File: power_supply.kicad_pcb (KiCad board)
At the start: 2 copper layers, 85 x 56 mm, 24 parts, among them J1 12v, 2A, J2 Screw_Terminal_01x02, J3 Fan, J4 Conn_01x05, M1 U3V70F5, M2 D24V50F5, U1 ALD910027, U2 MCP9700A-E_TO, U3 PIC12F1840-ISN

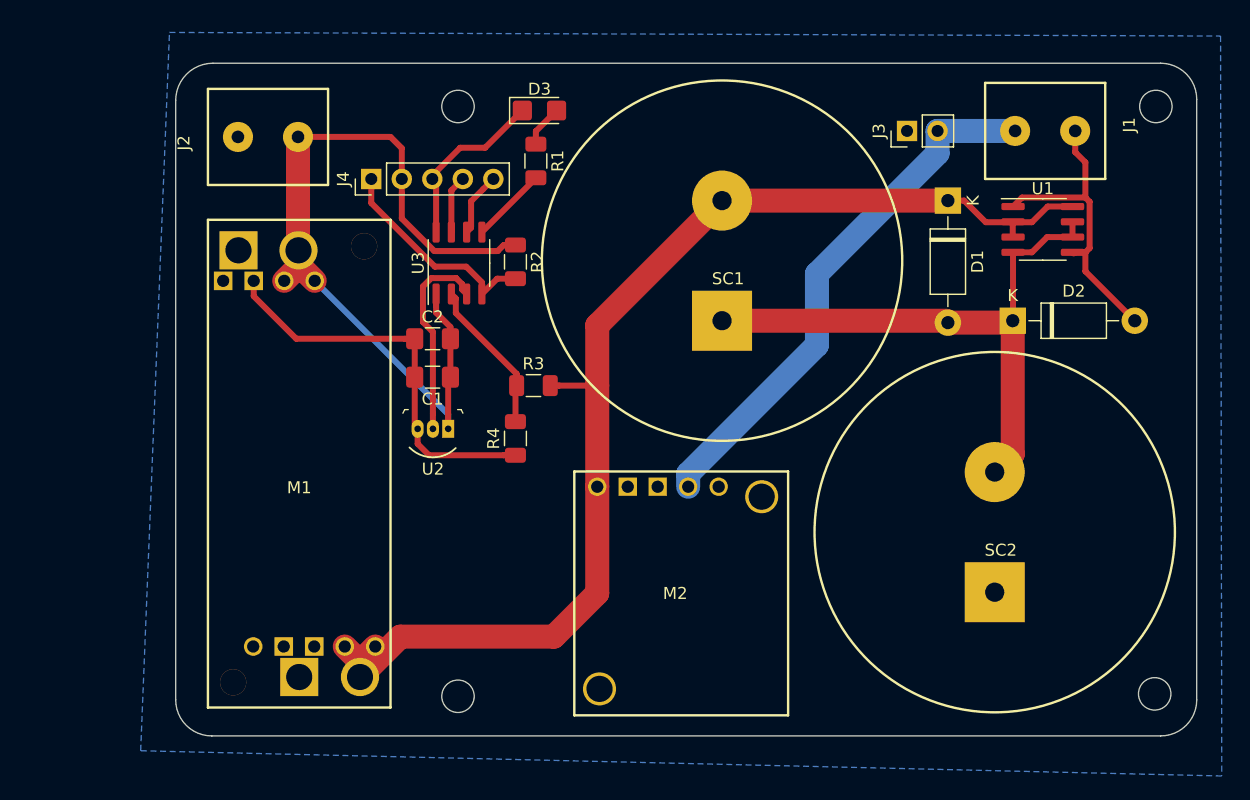
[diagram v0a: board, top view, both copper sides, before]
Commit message: Version 1.0 includes fixes/changes and FRAM support
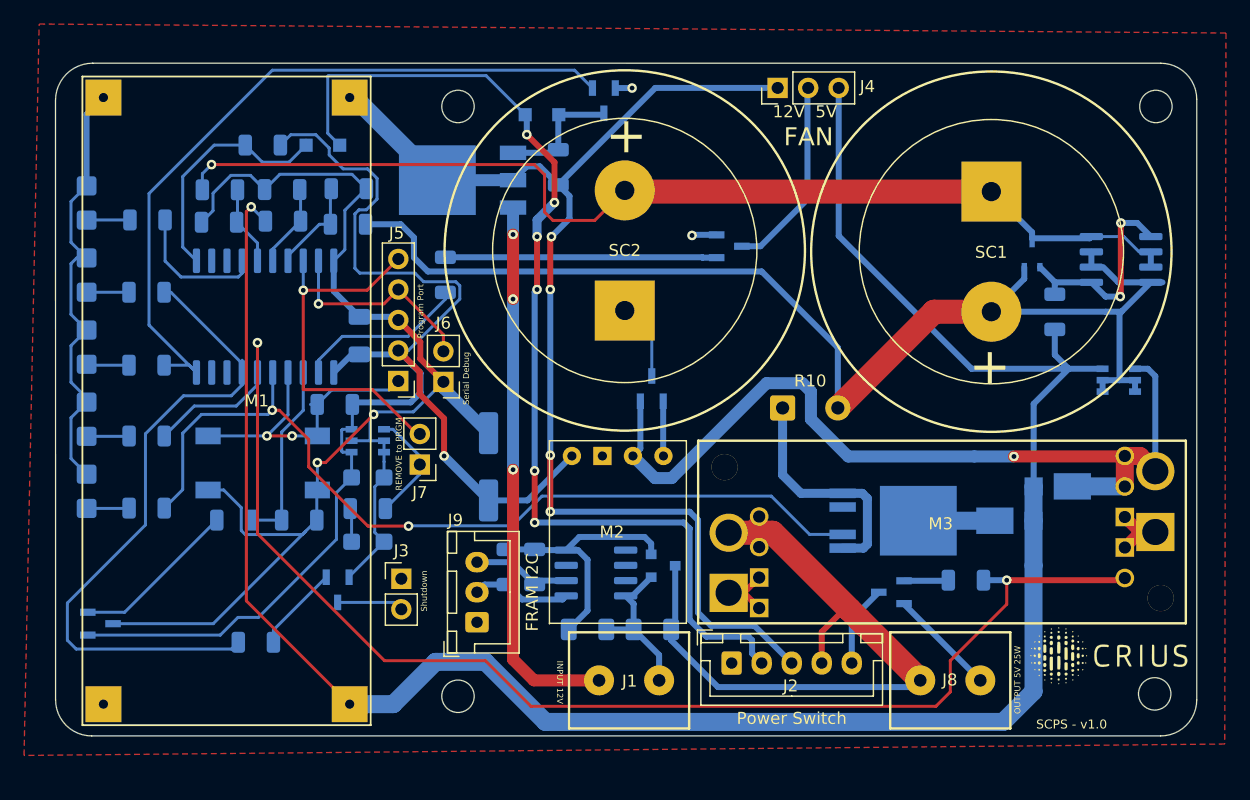
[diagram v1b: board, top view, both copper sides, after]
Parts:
- added C3: 2.2uF Tant, Capacitor_Tantalum_SMD:CP_EIA-3216-18_Kemet-A, B.Cu at (118.4, 115.8)
- added C4: 2.2uF Tant, Capacitor_Tantalum_SMD:CP_EIA-3216-18_Kemet-A, B.Cu at (118.4, 121.2)
- added C5: 1uF, Capacitor_SMD:C_1206_3216Metric_Pad1.33x1.80mm_HandSolder, B.Cu at (136.7, 128.5)
- added C6: 1uF, Capacitor_SMD:C_1206_3216Metric_Pad1.33x1.80mm_HandSolder, B.Cu at (142.1, 128.5)
- added D10: PWRUP, Diode_SMD:D_1206_3216Metric_Castellated, B.Cu at (95.0, 111.0)
- added D4: FAULT, Diode_SMD:D_1206_3216Metric_Castellated, B.Cu at (95.0, 117.0)
- added D5: V8PAM10S, Footprint_Library:DO-221BC, B.Cu at (171.8, 119.5)
- added D6: MAINPWR, Diode_SMD:D_1206_3216Metric_Castellated, B.Cu at (95.0, 105.0)
- added D7: BAT54SW, Package_TO_SOT_SMD:SOT-323_SC-70, B.Cu at (173.7, 97.3)
- added D8: Activity, Diode_SMD:D_1206_3216Metric_Castellated, B.Cu at (95.0, 93.0)
- added D9: V8PAM10S, Footprint_Library:DO-221BC, B.Cu at (175.8, 116.6)
- added G***: LOGO, Crius:Crius_logo_36x9mm, B.Cu at (170.4, 86.8)
- added G***: LOGO, Crius:Crius_logo_20x5mm, F.Cu at (180.1, 130.7)
- added J5: Program, Connector_PinHeader_2.54mm:PinHeader_1x05_P2.54mm_Vertical, F.Cu at (121.0, 107.8)
- added J6: Serial Debug, Connector_PinHeader_2.54mm:PinHeader_1x02_P2.54mm_Vertical, F.Cu at (124.7, 107.9)
- added J7: REMOVE to PRGM, Connector_PinHeader_2.54mm:PinHeader_1x02_P2.54mm_Vertical, F.Cu at (122.7, 114.8)
- added J8: 5V 25W, Connectors:Screw_Terminal_2Pin, F.Cu at (166.9, 132.7)
- added J9: FRAM I2C, Connector_JST:JST_XH_B3B-XH-A_1x03_P2.50mm_Vertical, F.Cu at (127.5, 127.9)
- added M3: U3V70F5, Pololu:U3V70F5, F.Cu at (166.2, 120.4)
- added Q1: BSS806, digikey-footprints:SOT-23-3, B.Cu at (138.1, 84.5)
- added Q2: BSS806, digikey-footprints:SOT-23-3, B.Cu at (148.5, 96.6)
- added Q3: SPD18P06PGBTMA1, Package_TO_SOT_SMD:TO-252-3_TabPin2, B.Cu at (126.3, 91.1)
- added Q4: BSS806, digikey-footprints:SOT-23-3, B.Cu at (162.0, 125.4)
- added Q5: BSS806, digikey-footprints:SOT-23-3, B.Cu at (115.9, 125.2)
- added Q6: SQ3495-EV, digikey-footprints:SOT-23-6, B.Cu at (180.9, 107.8)
- added R10: 1R 25W, Connector_Wire:SolderWire-0.5sqmm_1x02_P4.6mm_D0.9mm_OD2.1mm, F.Cu at (152.9, 110.1)
- added R11: 1k, Resistor_SMD:R_1206_3216Metric, B.Cu at (100.0, 106.5)
- added R12: 10k, Resistor_SMD:R_1206_3216Metric, B.Cu at (109.7, 88.2)
- added R13: 9k 0.1%, Resistor_SMD:R_1206_3216Metric, B.Cu at (106.1, 91.9)
- added R14: 1k, Resistor_SMD:R_1206_3216Metric, B.Cu at (100.1, 94.4)
- added R15: 9k 0.1%, Resistor_SMD:R_1206_3216Metric, B.Cu at (111.3, 94.5)
- added R16: 1k 0.1%, Resistor_SMD:R_1206_3216Metric, B.Cu at (106.0, 94.6)
- added R17: 9k 0.1%, Resistor_SMD:R_1206_3216Metric, B.Cu at (116.8, 94.8)
- added R18: 10k, Resistor_SMD:R_1206_3216Metric, B.Cu at (175.6, 102.1)
- added R19: 1k 0.1%, Resistor_SMD:R_1206_3216Metric, B.Cu at (111.3, 91.9)
- added R20: 1k 0.1%, Resistor_SMD:R_1206_3216Metric, B.Cu at (116.8, 91.8)
- added R21: 1k, Resistor_SMD:R_1206_3216Metric, B.Cu at (100.0, 112.4)
- added R22: 50, Resistor_SMD:R_1206_3216Metric, B.Cu at (118.4, 118.4)
- added R23: 10k, Resistor_SMD:R_1206_3216Metric, B.Cu at (132.3, 123.3)
- added R24: 10k, Resistor_SMD:R_1206_3216Metric, B.Cu at (130.0, 123.3)
- added R5: 1k, Resistor_SMD:R_1206_3216Metric, B.Cu at (168.2, 124.4)
- added R6: 1k, Resistor_SMD:R_1206_3216Metric, B.Cu at (100.0, 118.4)
- added R7: 1k 0.1%, Resistor_SMD:R_1206_3216Metric, B.Cu at (107.3, 119.4)
- added R8: 1k 0.1%, Resistor_SMD:R_1206_3216Metric, B.Cu at (112.7, 119.4)
- added R9: 10k, Resistor_SMD:R_1206_3216Metric, B.Cu at (115.7, 109.8)
- added S1: RESET, digikey-footprints:Switch_Tactile_SMD_6x6mm, B.Cu at (109.7, 114.6)
- added U4: PIC16F1709, Package_SO:SOIC-20W_7.5x12.8mm_P1.27mm, B.Cu at (109.9, 102.5)
- added U5: MCP111-195, digikey-footprints:SOT-23-3, B.Cu at (142.1, 108.5)
- added U6: MB85RC1MT, Package_SO:SOIC-8_3.9x4.9mm_P1.27mm, B.Cu at (137.4, 123.8)
- added U7: MCP1700-3302E_SOT23, Package_TO_SOT_SMD:SOT-23, B.Cu at (143.0, 123.2)
- added VRef1: MCP1501-6Pin, digikey-footprints:SOT-23-6, B.Cu at (118.4, 112.8)
- C1: value .1 -> 100uF; footprint Capacitor_SMD:C_1206_3216Metric_Pad1.42x1.75mm_HandSolder -> Capacitor_SMD:CP_Elec_6.3x5.2; moved to B.Cu
- C2: footprint Capacitor_SMD:C_1206_3216Metric_Pad1.42x1.75mm_HandSolder -> Capacitor_SMD:C_1206_3216Metric_Pad1.33x1.80mm_HandSolder; moved to B.Cu
- D1, D2: value 1N5817 -> 1N914; footprint Diode_THT:D_DO-41_SOD81_P10.16mm_Horizontal -> Diode_SMD:D_SOD-123F; moved to B.Cu
- D3: value LED -> ShutDown; moved to B.Cu
- J1: value 12v, 2A -> 12v, 0.5A nominal, 5A Surge
- J2: value Screw_Terminal_01x02 -> Power Switch; footprint Connectors:Screw_Terminal_2Pin -> Connector_JST:JST_XH_B5B-XH-A_1x05_P2.50mm_Vertical
- J3: value Fan -> Shutdown
- J4: value Conn_01x05 -> 12V 5V; footprint Connector_PinHeader_2.54mm:PinHeader_1x05_P2.54mm_Vertical -> Connector_PinHeader_2.54mm:PinHeader_1x03_P2.54mm_Vertical
- M1: value U3V70F5 -> XL4015; footprint Pololu Regulators:U3V70F5 -> Footprint_Library:XL4015
- M2: value D24V50F5 -> U1V11F5; footprint Pololu Regulators:D24V50F5 -> Pololu:U1V11Fx
- R1: value 1k -> 10k; moved to B.Cu
- R2: value 10k -> 1k; moved to B.Cu
- R3, R4: moved to B.Cu
- SC1, SC2: value SuperCap -> 100F/200F; footprint SuperCaps:SCC-30mm -> SuperCaps:SCC-22-30mm
- U1: value ALD910027 -> MCP9700A; footprint Package_SO:SOIC-8_3.9x4.9mm_P1.27mm -> digikey-footprints:SOT-23-3; moved to B.Cu
- U2: value MCP9700A-E_TO -> BTS443P; footprint digikey-footprints:TO-92-3 -> Package_TO_SOT_SMD:TO-252-4; moved to B.Cu
- U3: value PIC12F1840-ISN -> ALD910027; footprint Package_SO:SO-8_3.9x4.9mm_P1.27mm -> Package_SO:SOIC-8_3.9x4.9mm_P1.27mm; moved to B.Cu
- moved U1 85.0 mm to (96.2, 128.0)
- moved J2 58.4 mm to (148.7, 131.3), turned to 0 degrees
- moved J1 57.4 mm to (140.2, 132.7)
- moved J3 56.2 mm to (121.2, 124.3), turned to 0 degrees
- moved U3 55.1 mm to (181.1, 97.7), turned to 0 degrees
- moved D1 52.2 mm to (114.7, 88.2), turned to 180 degrees
- moved D2 42.8 mm to (132.9, 85.7)
- moved D3 40.1 mm to (95.0, 99.0), turned to 270 degrees
- moved SC2 38.7 mm to (139.8, 97.0)
- moved R2 38.3 mm to (109.1, 129.6), turned to 0 degrees
- moved U2 37.8 mm to (162.1, 119.5), turned to 0 degrees
- moved J4 34.7 mm to (152.5, 83.4)
- moved R3 33.1 mm to (100.0, 100.4), turned to 180 degrees
- moved SC1 22.4 mm to (170.3, 97.0), turned to 180 degrees
- moved R4 14.8 mm to (124.9, 99.0)
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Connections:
- C1 pad 1: /5V -> Net-(C1-Pad1)
- C1 pad 2: /GND -> Net-(C1-Pad2)
- C2 pad 1: /GND -> Net-(C1-Pad2)
- C2 pad 2: /5V -> Net-(C1-Pad1)
- D1 pad 1: /2.5-5V -> Net-(D1-Pad1)
- D2 pad 1: Net-(D1-Pad2) -> Net-(D1-Pad1)
- D2 pad 2: /GND -> Net-(D2-Pad2)
- D3 pad 1: /GND -> Net-(C1-Pad2)
- J1 pad 1: /GND -> Net-(C1-Pad2)
- J1 pad 2: /12v -> Net-(J1-Pad2)
- J2 pad 1: /GND -> Net-(C1-Pad2)
- J2 pad 2: /5V -> Net-(D1-Pad1)
- J3 pad 1: /GND -> Net-(C1-Pad2)
- J3 pad 2: /12v -> Net-(J3-Pad2)
- J4 pad 1: Net-(J4-Pad1) -> Net-(J2-Pad3)
- J4 pad 2: /5V -> Net-(J4-Pad2)
- J4 pad 3: /GND -> Net-(D5-Pad2)
- M1 pad 1: Net-(M1-Pad1) -> Net-(J2-Pad3)
- M1 pad 2: /GND -> Net-(C1-Pad2)
- M1 pad 3: /GND -> Net-(C1-Pad2)
- M1 pad 4: /GND -> Net-(D5-Pad2)
- M2 pad 1: Net-(M2-Pad1) -> Net-(C1-Pad1)
- M2 pad 2: /12v -> Net-(C1-Pad2)
- M2 pad 3: /GND -> Net-(D9-Pad1)
- M2 pad 4: /GND -> Net-(M2-Pad4)
- R1 pad 1: Net-(D3-Pad2) -> Net-(D2-Pad2)
- R1 pad 2: Net-(R1-Pad2) -> Net-(J2-Pad3)
- R2 pad 1: /5V -> Net-(R2-Pad1)
- R2 pad 2: Net-(J4-Pad1) -> Net-(Q5-Pad1)
- R3 pad 1: Net-(R3-Pad1) -> Net-(R2-Pad1)
- R3 pad 2: /2.5-5V -> Net-(D3-Pad2)
- R4 pad 1: /GND -> Net-(R4-Pad1)
- R4 pad 2: Net-(R3-Pad1) -> Net-(Q2-Pad1)
- SC1 pad 1: Net-(D1-Pad2) -> Net-(D7-Pad3)
- SC1 pad 2: /2.5-5V -> Net-(D7-Pad2)
- SC2 pad 1: /GND -> Net-(C1-Pad2)
- SC2 pad 2: Net-(D1-Pad2) -> Net-(D7-Pad3)
- U1 pad 1: /GND -> Net-(C1-Pad1)
- U1 pad 2: /2.5-5V -> Net-(R7-Pad2)
- U1 pad 3: /2.5-5V -> Net-(C1-Pad2)
- U2 pad 1: /5V -> Net-(R10-Pad1)
- U2 pad 2: Net-(U2-Pad2) -> Net-(R6-Pad1)
- U2 pad 3: /GND -> Net-(D5-Pad1)
- U3 pad 1: /5V -> Net-(C1-Pad2)
- U3 pad 2: Net-(R3-Pad1) -> Net-(D7-Pad2)
- U3 pad 3: Net-(U2-Pad2) -> Net-(D7-Pad2)
- U3 pad 4: Net-(J4-Pad1) -> Net-(D7-Pad3)
- U3 pad 5: Net-(R1-Pad2) -> Net-(C1-Pad2)
- U3 pad 6: Net-(J4-Pad5) -> Net-(D7-Pad3)
- U3 pad 7: Net-(J4-Pad4) -> Net-(D7-Pad3)
- U3 pad 8: /GND -> Net-(D7-Pad2)
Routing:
- net Net-(C1-Pad2): track 0.00 -> 214.2 mm, vias 0 -> 6
- net Net-(D5-Pad2): track 0.00 -> 179.0 mm, vias 0 -> 1
- net Net-(M3-Pad1): track 0.00 -> 116.2 mm, vias 0 -> 2
- net Net-(C1-Pad1): track 0.00 -> 115.9 mm, vias 0 -> 1
- net Net-(D7-Pad2): track 0.00 -> 102.9 mm
- net Net-(J2-Pad3): track 0.00 -> 101.0 mm, vias 0 -> 4
- net /2.5-5V: track 100.2 -> 0.00 mm
- net Net-(D7-Pad3): track 0.00 -> 89.6 mm, vias 0 -> 1
- net Net-(D1-Pad1): track 0.00 -> 88.5 mm, vias 0 -> 6
- net Net-(R6-Pad1): track 0.00 -> 74.6 mm, vias 0 -> 2
- net /GND: track 73.8 -> 0.00 mm
- net Net-(D9-Pad1): track 0.00 -> 73.5 mm, vias 0 -> 1
- net /5V: track 70.0 -> 0.00 mm
- net Net-(C6-Pad1): track 0.00 -> 61.8 mm
- net Net-(Q1-Pad1): track 0.00 -> 61.3 mm
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- added copper zone on F.Cu, net Net-(C1-Pad2)
- removed copper zone on B.Cu, net /GND
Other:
- board size 85 x 56 mm -> 95 x 56 mm
- board text added: "- 12V +"
- board text added: "- 5V +"
- board text added: "FAN"
- board text added: "INPUT 12V"
- board text added: "INPUT PWR"
- board text added: "LED|5V|12V|SW|GND"
- board text added: "OUTPUT 5V 25W"
- board text added: "OUTPUT PWR"
- board text added: "POWER SW"
- board text added: "Program Port"
- board text added: "SCPS - v1.0"
